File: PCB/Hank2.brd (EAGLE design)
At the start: 256.5 x 129.5 mm, 114 parts, among them IC3 ATMEGA328-20P, T1 2n2222, T2 2n2222, T3 2n2222, T4 2n2222, T5 2n2222, T6 2n2222, T7 2n2222, T8 2n2222

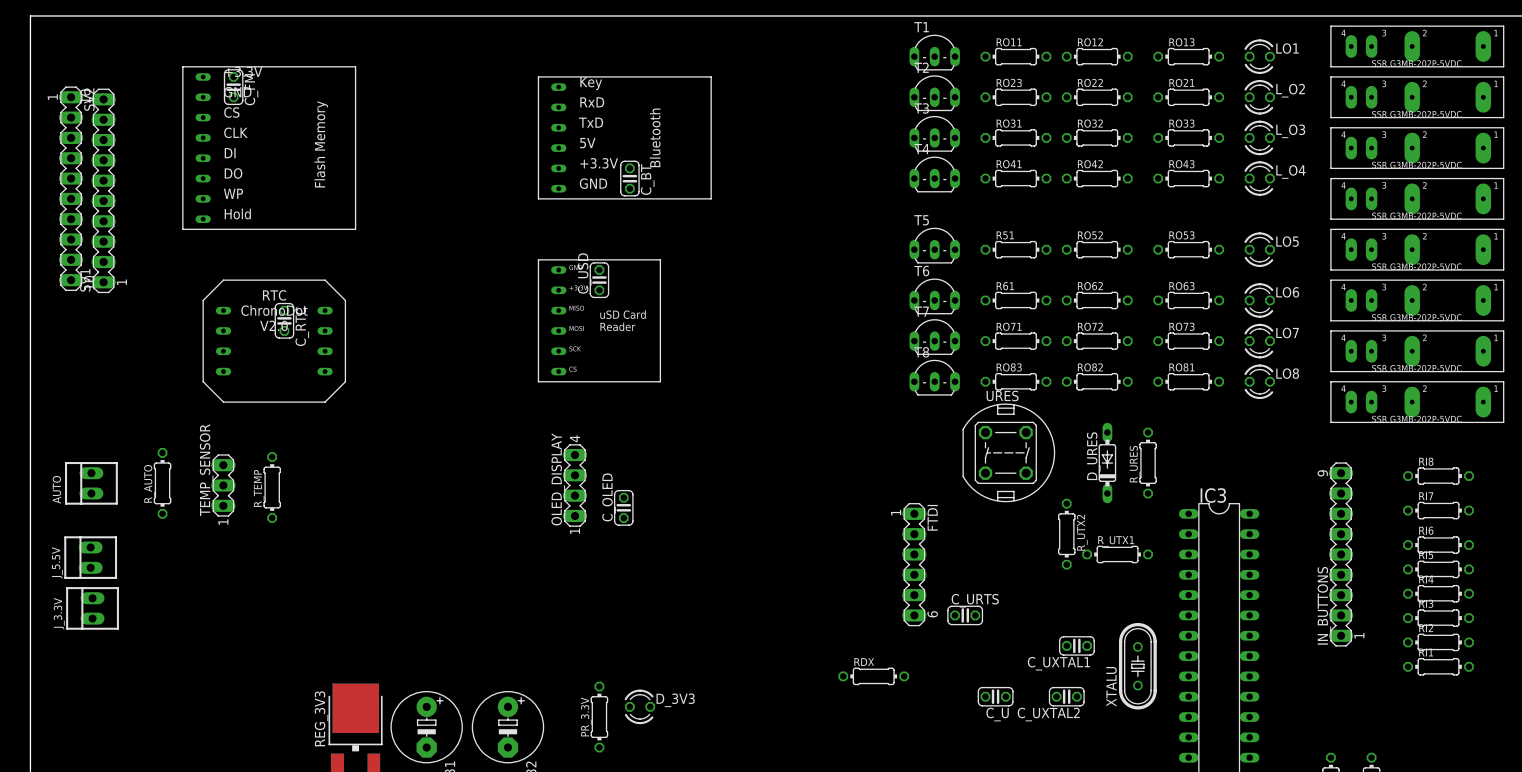
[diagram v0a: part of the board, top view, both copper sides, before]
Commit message: Added parts schedule
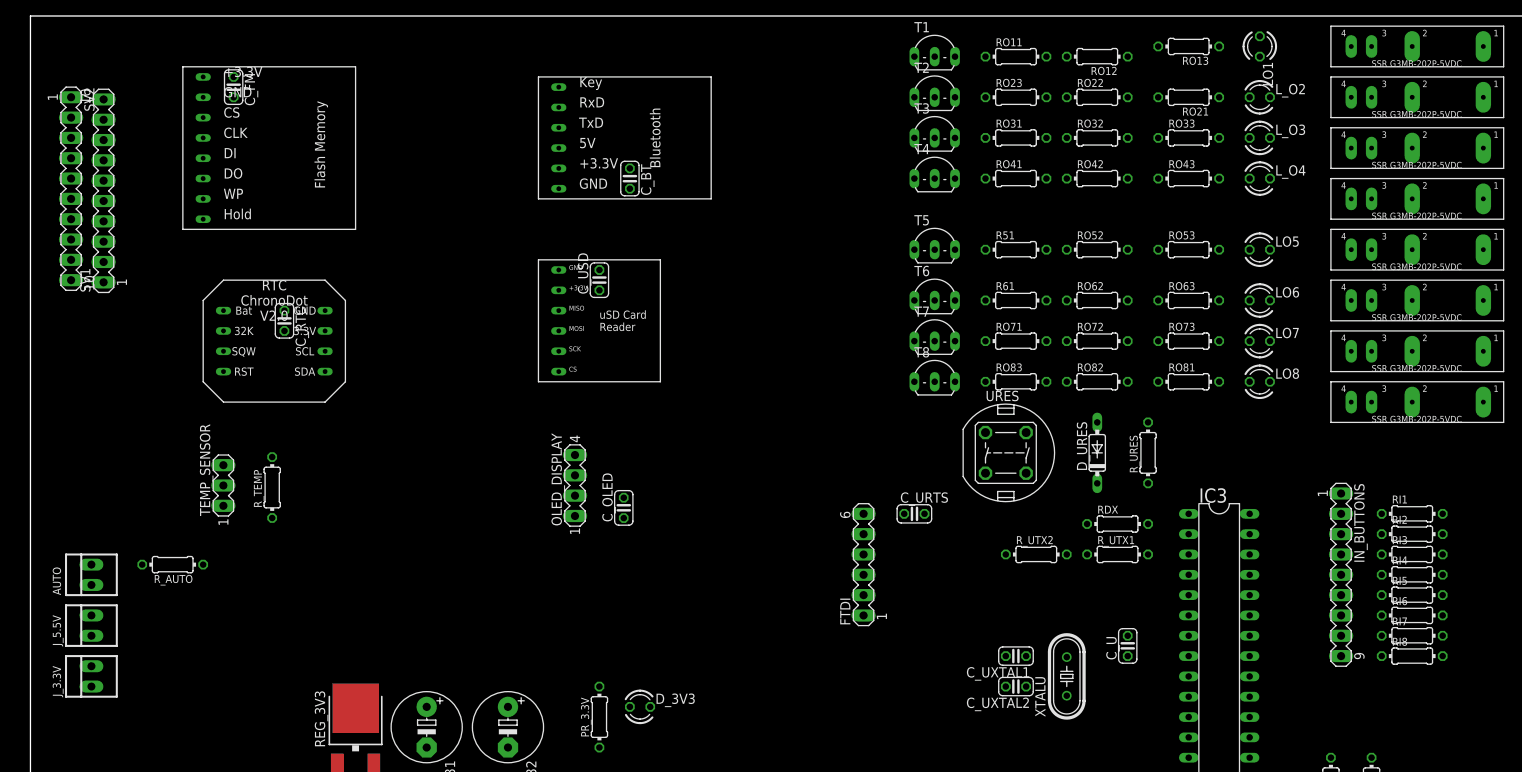
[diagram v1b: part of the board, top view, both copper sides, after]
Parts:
- IN_BUTTONS: value (none) -> User Inputs
- RI8, R_AUTO: value (none) -> 330
- RO33: value (none) -> 1k
- X1: value (none) -> Sockets 1
- X2: value (none) -> Sockets 2
- moved RDX 35.9 mm to (135.9, 66.0)
- moved RI8 22.7 mm to (172.7, 49.5)
- moved RI1 19.4 mm to (172.7, 67.3)
- moved C_U 17.7 mm to (137.2, 50.8), turned to 90 degrees
- moved RI7 16.0 mm to (172.7, 52.1)
- moved C_URTS 14.2 mm to (110.5, 67.3)
- moved RI2 13.9 mm to (172.7, 64.8)
- moved AUTO 11.4 mm to (7.62, 59.7)
- moved R_AUTO 10.2 mm to (17.8, 61.0), turned to 180 degrees
- moved RI6 9.39 mm to (172.7, 54.6)
- moved XTALU 8.98 mm to (129.5, 47.0)
- moved RI3 8.61 mm to (172.7, 62.2)
- moved J_3.3V 8.50 mm to (7.62, 47.0)
- moved J_5.5V 8.50 mm to (7.62, 53.3)
- moved C_UXTAL1 7.73 mm to (123.2, 49.5)
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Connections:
- removed net N$10: U$4.KEY
- removed net N$13: U$4.5V
- removed net N$15: R51.2, RO52.2
- removed net N$19: R61.2, RO62.2
- removed net N$24: RO71.2, RO72.2
- removed net N$28: RO81.2, RO82.2
- removed net N$36: RO21.2, RO22.2
- removed net N$40: RO31.2, RO32.2
- removed net N$44: RO41.2, RO42.2
- removed net N$7: RI1.2, RI2.2, RI3.2, RI4.2, RI5.2, RI6.2, RI7.2, RI8.2
- removed net RXD: RDX.2
- removed net SERIAL_RXD: U$4.RXD
- removed net SERIAL_TXD: U$4.TXD
- removed net TXD: FTDI.4
- new net BT_RX: SV1.4, U$4.RXD
- new net BT_TX: SV1.5, U$4.TXD
- net GND: now also RI1.2, RI2.2, RI3.2, RI4.2, RI5.2, RI6.2, RI7.2, RI8.2; no longer SV1.4, SV1.5
- net IN1: now also IC3.18, IN_BUTTONS.9, RI8.1; no longer IC3.23, IN_BUTTONS.2, RI1.1
- net IN2: now also IC3.19, IN_BUTTONS.8, RI7.1; no longer IC3.24, IN_BUTTONS.3, RI2.1
- net IN3: now also IC3.23, IN_BUTTONS.7, RI6.1; no longer IC3.25, IN_BUTTONS.4, RI3.1
- net IN4: now also IC3.24, IN_BUTTONS.6, RI5.1; no longer IC3.26, IN_BUTTONS.5, RI4.1
- net IN5: now also IC3.25, IN_BUTTONS.5, RI4.1; no longer IC3.27, IN_BUTTONS.6, RI5.1
- net IN6: now also IC3.26, IN_BUTTONS.4, RI3.1; no longer IC3.28, IN_BUTTONS.7, RI6.1
- net IN7: now also IC3.27, IN_BUTTONS.3, RI2.1; no longer IC3.18, IN_BUTTONS.8, RI7.1
- net IN8: now also IC3.28, IN_BUTTONS.2, RI1.1; no longer IC3.19, IN_BUTTONS.9, RI8.1
- net OUT2: now also RO21.2, RO22.2
- net OUT3: now also RO31.2, RO32.2
- net OUT4: now also RO41.2, RO42.2
- net OUT5: now also R51.2, RO52.2
- net OUT6: now also R61.2, RO62.2
- net OUT7: now also RO71.2, RO72.2
- net OUT8: now also RO81.2, RO82.2
- net U_RX: now also FTDI.4
- net U_TX: now also RDX.2

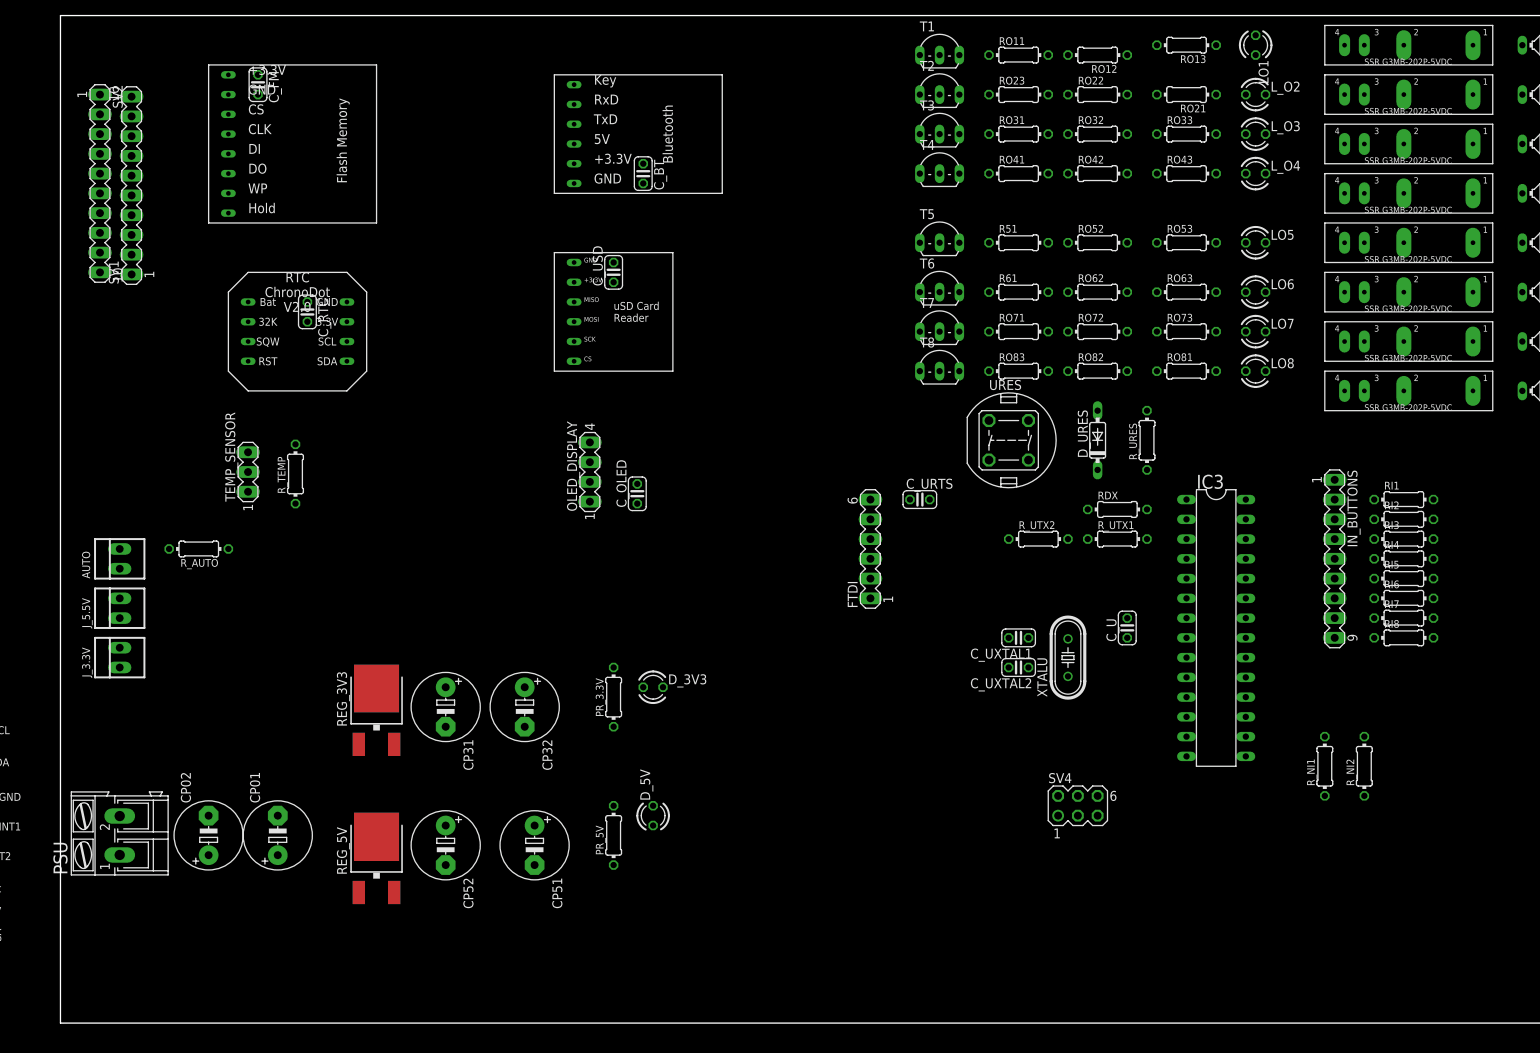
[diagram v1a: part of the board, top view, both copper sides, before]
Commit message: Updating parts footprint in the brd
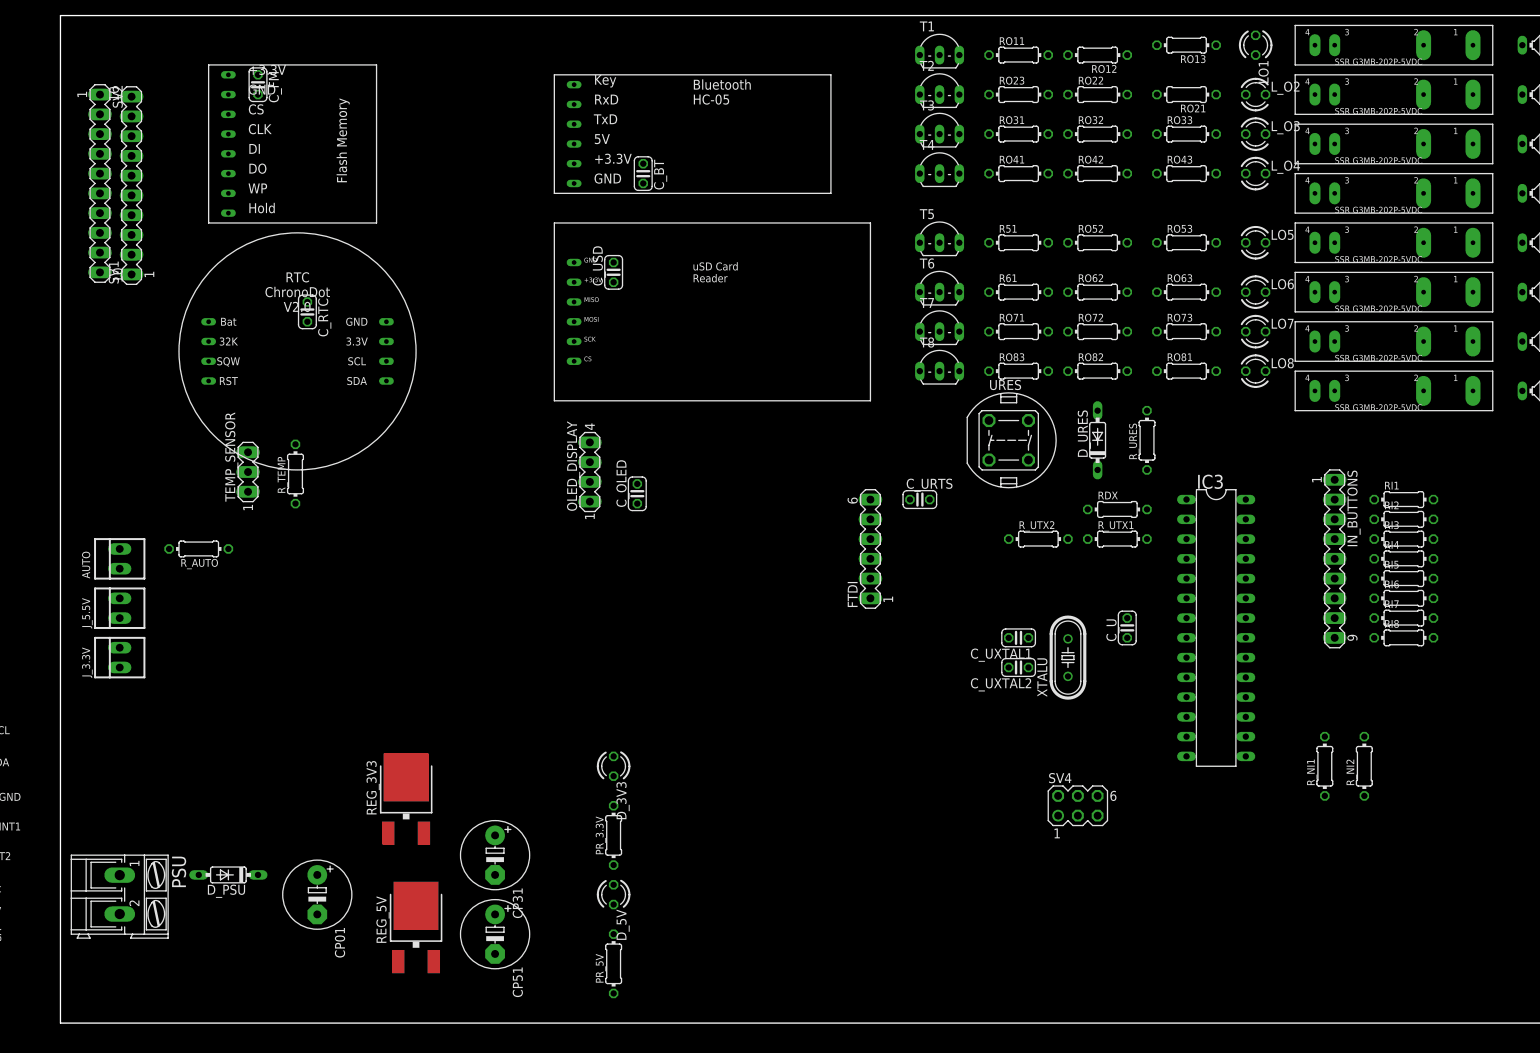
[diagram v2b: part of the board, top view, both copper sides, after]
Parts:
- removed CP02, CP32, CP52: 100n, rcl:E5-8,5
- added D_PSU: 1N4148DO35-7, diode:DO35-7
- CP31, CP51: value 100u -> 22uF
- moved CP31 20.1 mm to (55.9, 21.6)
- moved PR_3.3V 17.8 mm to (71.1, 24.1)
- moved PR_5V 16.5 mm to (71.1, 7.62)
- moved U$7 12.8 mm to (83.8, 91.4)
- moved CP51 12.5 mm to (55.9, 11.4)
- moved REG_3V3 12.0 mm to (44.5, 29.2)
- moved D_5V 11.4 mm to (71.1, 16.5), turned to 270 degrees
- moved D_3V3 11.4 mm to (71.1, 33.0), turned to 270 degrees
- moved REG_5V 10.2 mm to (45.7, 12.7)
- moved CP01 9.16 mm to (33.0, 16.5), turned to 270 degrees
- moved PSU 7.62 mm to (7.62, 16.5), turned to 270 degrees
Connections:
- new net N$7: D_PSU.A, PSU.1
- net +3V3: no longer CP32.+
- net +5V: no longer CP52.+
- net CP12: now also D_PSU.C; no longer CP02.+, PSU.1
- net GND: no longer CP02.-, CP32.-, CP52.-
